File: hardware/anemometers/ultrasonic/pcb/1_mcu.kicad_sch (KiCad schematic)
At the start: 59 parts, among them Q1 SI2301CDS-T1-GE3, SW1 B3U-1000P, U1 TCAN330GDCNR, U12 Sort_Symbol, U14 Sort_Symbol, U15 Sort_Symbol, U16 Sort_Symbol, U2 STM32L476RGT6, U3 XC6206P332MR, X1 32.768KHz, X2 25M

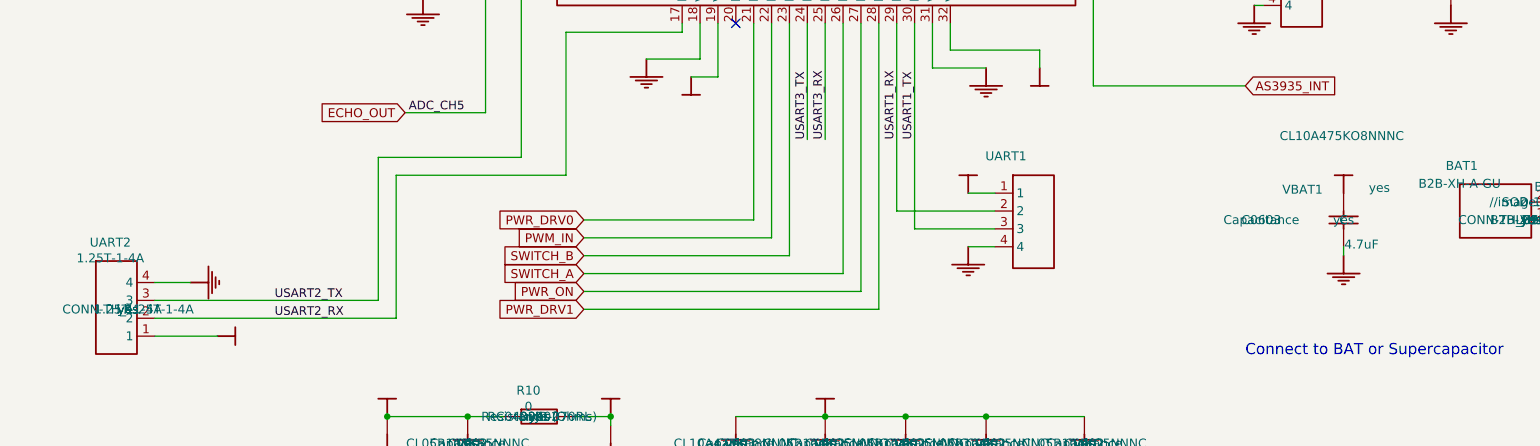
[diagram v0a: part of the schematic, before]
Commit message: Fix mux
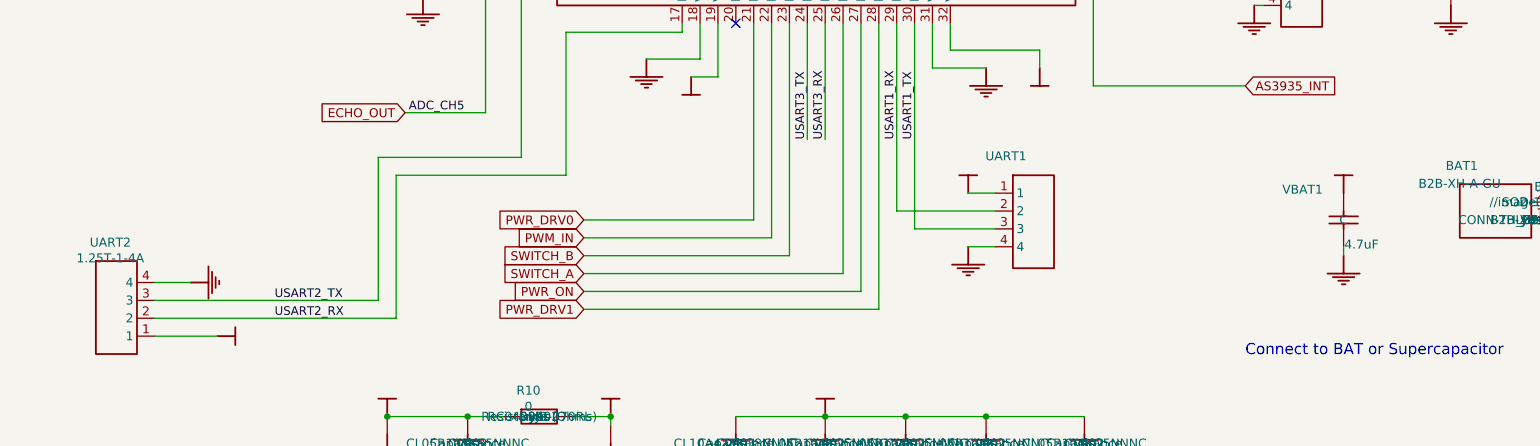
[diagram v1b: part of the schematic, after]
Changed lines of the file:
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@@
 					(size 1.27 1.27)
 				)
+				(hide yes)
 			)
 		)
@@
 					(size 1.27 1.27)
 				)
+				(hide yes)
 			)
 		)
@@
 					(size 1.27 1.27)
 				)
+				(hide yes)
 			)
 		)
@@
 					(size 1.27 1.27)
 				)
+				(hide yes)
 			)
 		)
@@
 					(size 1.27 1.27)
 				)
+				(hide yes)
 			)
 		)
@@
 					(size 1.27 1.27)
 				)
+				(hide yes)
 			)
 		)
@@
 					(size 1.27 1.27)
 				)
+				(hide yes)
 			)
 		)
@@
 					(size 1.27 1.27)
 				)
+				(hide yes)
 			)
 		)
@@
 					(size 1.27 1.27)
 				)
+				(hide yes)
 			)
 		)
@@
 					(size 1.27 1.27)
 				)
+				(hide yes)
 			)
 		)
